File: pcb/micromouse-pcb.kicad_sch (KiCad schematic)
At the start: 42 parts, among them J1 Conn_01x06, J2 Conn_01x08, J3 Conn_01x08, M1 Motor_DC, Q1 BS170, Q2 TEFT4300, Q3 BS170, Q4 TEFT4300, Q5 BS170, Q6 TEFT4300, Q7 BS170, Q8 TEFT4300, SW1 SW_SPDT, U0 Teensy 4.1, U1 L7805, U2 DRV8833PWP

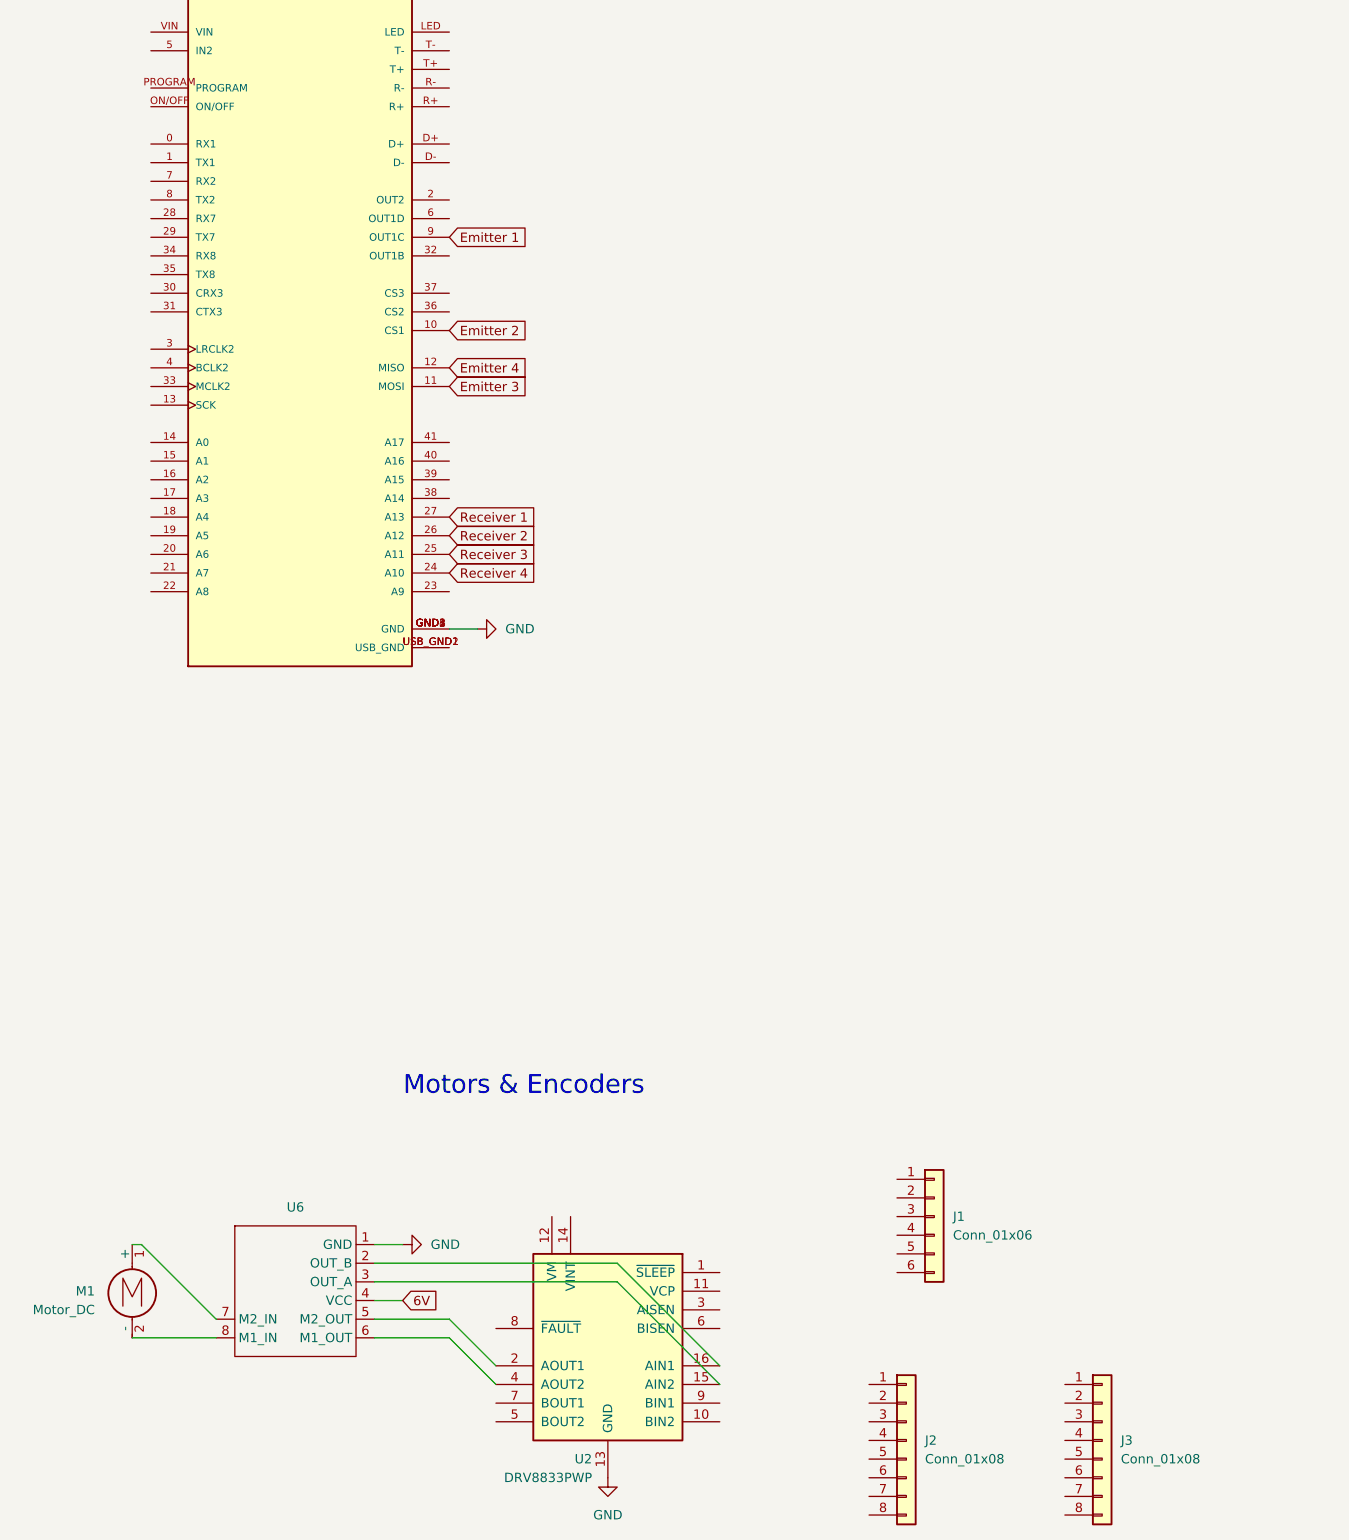
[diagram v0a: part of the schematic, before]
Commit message: worked a bit on motor module
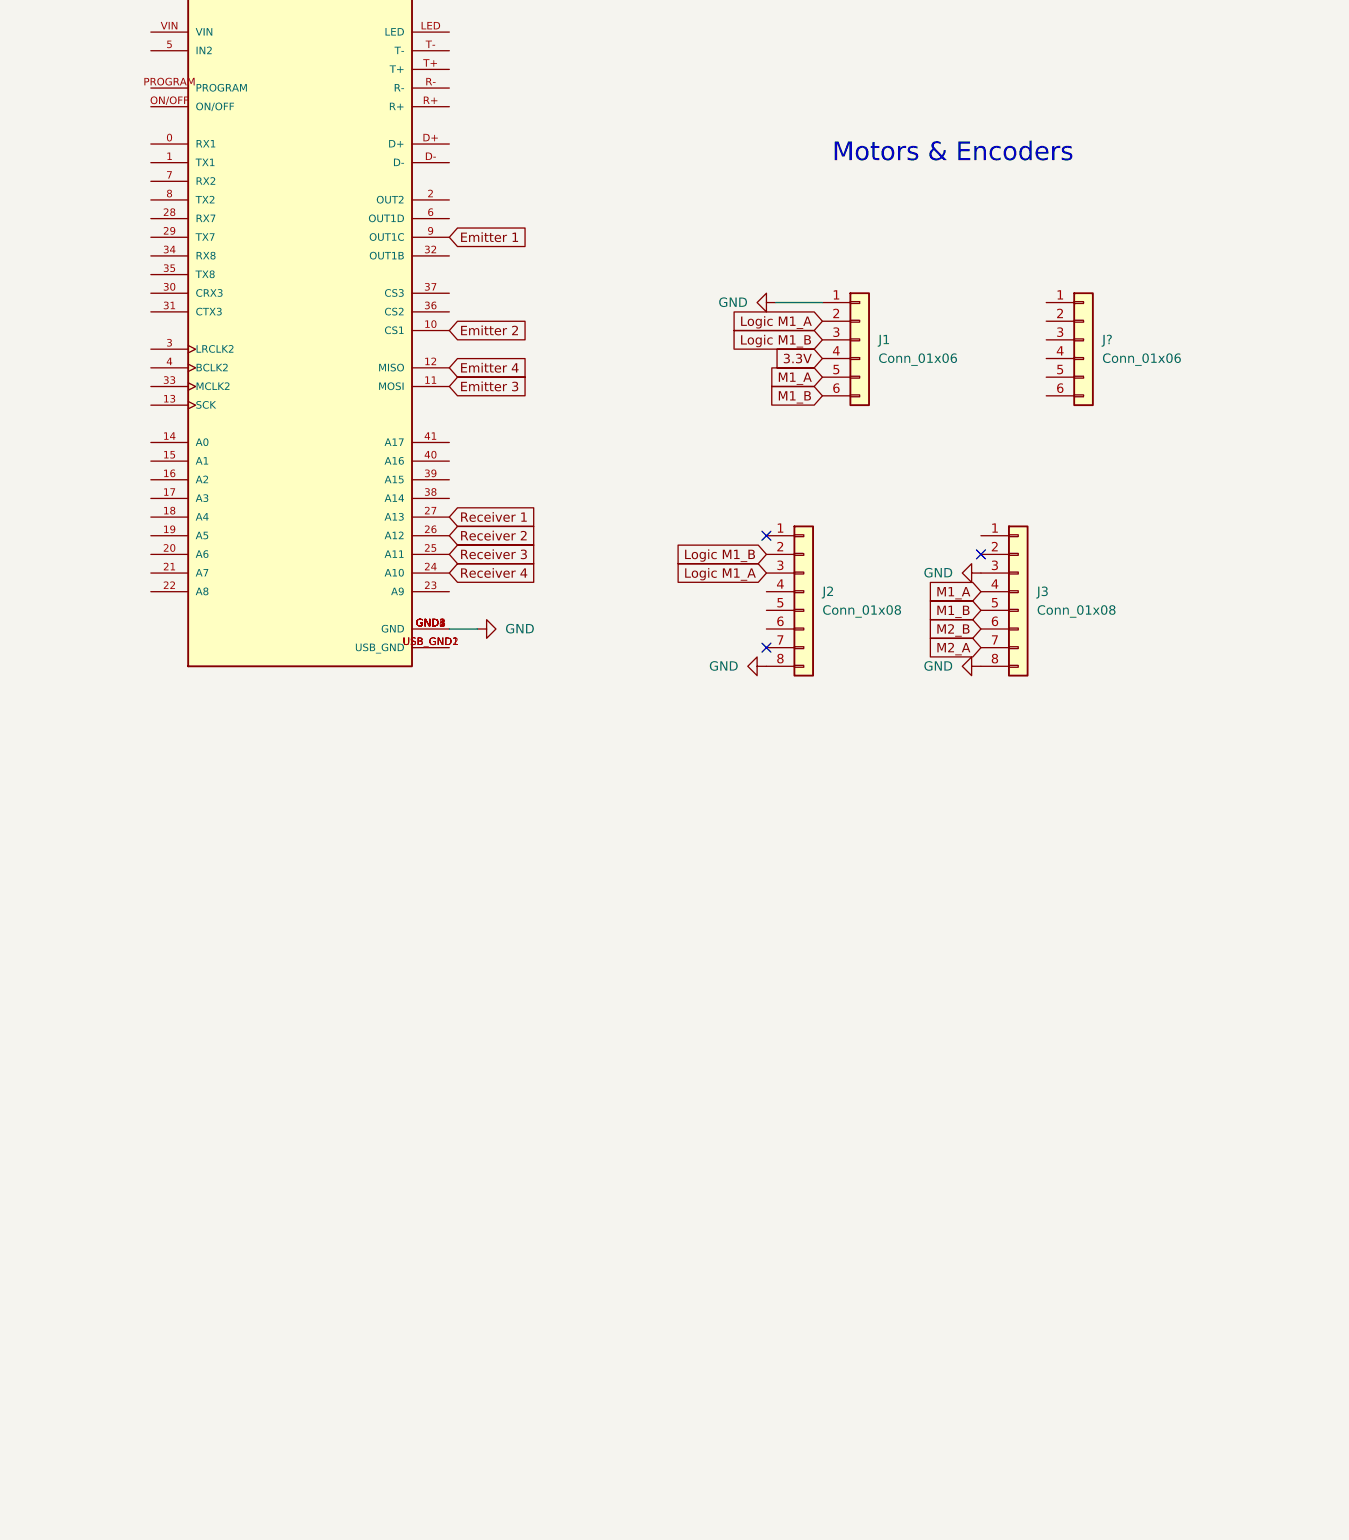
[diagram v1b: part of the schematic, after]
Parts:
- removed M1: Motor_DC, symbol Motor:Motor_DC
- removed U2: DRV8833PWP, Package_SO:HTSSOP-16-1EP_4.4x5mm_P0.65mm_EP3.4x5mm_Mask2.46x2.31mm_ThermalVias, symbol Driver_Motor:DRV8833PWP
- removed U6: ~, symbol micromouse-symbols:Polulu_Encoder
- added J?: Conn_01x06, symbol Connector_Generic:Conn_01x06
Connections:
- net 3.3V: now also J1.4 (Pin_4)
- net GND: now also J1.1 (Pin_1), J2.8 (Pin_8), J3.3 (Pin_3), J3.8 (Pin_8)
- net Logic M1_A: now reaches J1.2 (Pin_2)
- net Logic M1_A: now also J2.3 (Pin_3)
- net Logic M1_B: now reaches J1.3 (Pin_3)
- net Logic M1_B: now also J2.2 (Pin_2)
- net M1_A: now reaches J1.5 (Pin_5)
- net M1_A: now also J3.4 (Pin_4)
- net M1_B: now reaches J1.6 (Pin_6)
- net M1_B: now also J3.5 (Pin_5)
- net M2_B: now reaches J3.6 (Pin_6)
- net M2_A: now reaches J3.7 (Pin_7)
- no-connect marks 1 -> 4
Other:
- moved on the sheet: J1, J2, J3
